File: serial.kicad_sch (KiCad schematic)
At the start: 17 parts, among them U15 LM79L05AC, U3 AM26LV32, U5 AM26LV32, U6 AM26LS30, U7 AM26LS30, U8 Am85C80

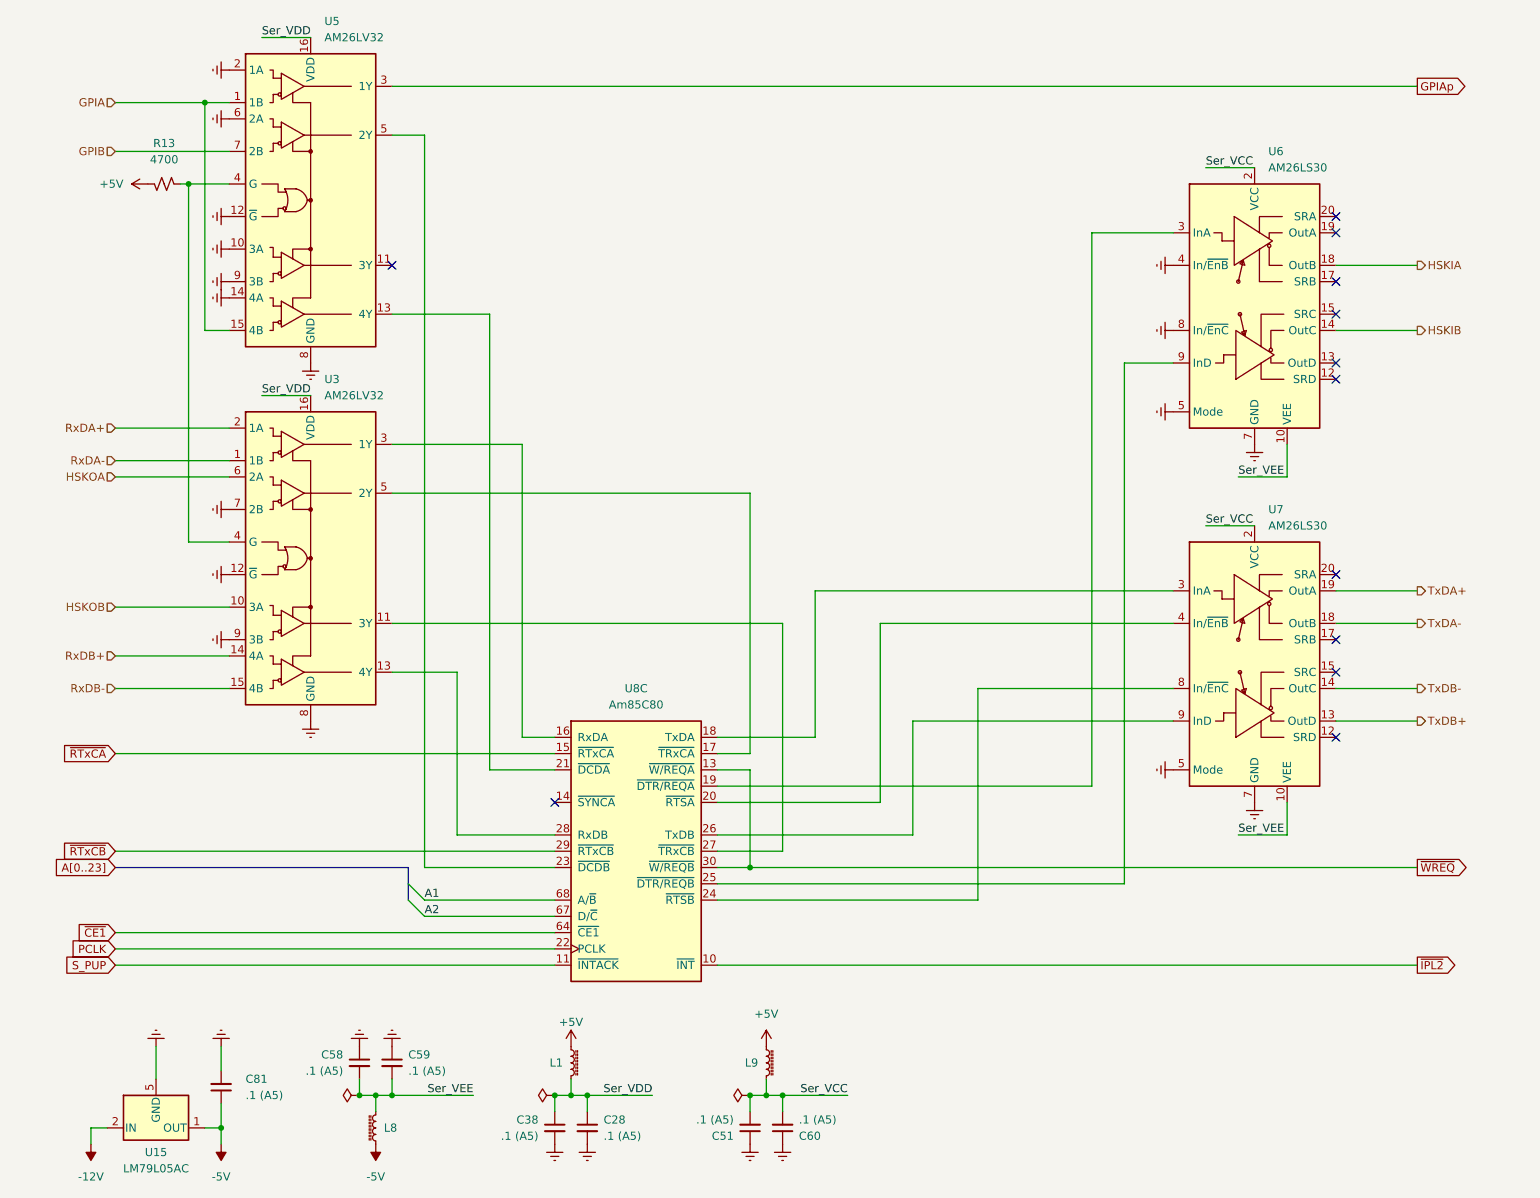
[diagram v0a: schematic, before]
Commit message: More cleanup and cosmetic fixes
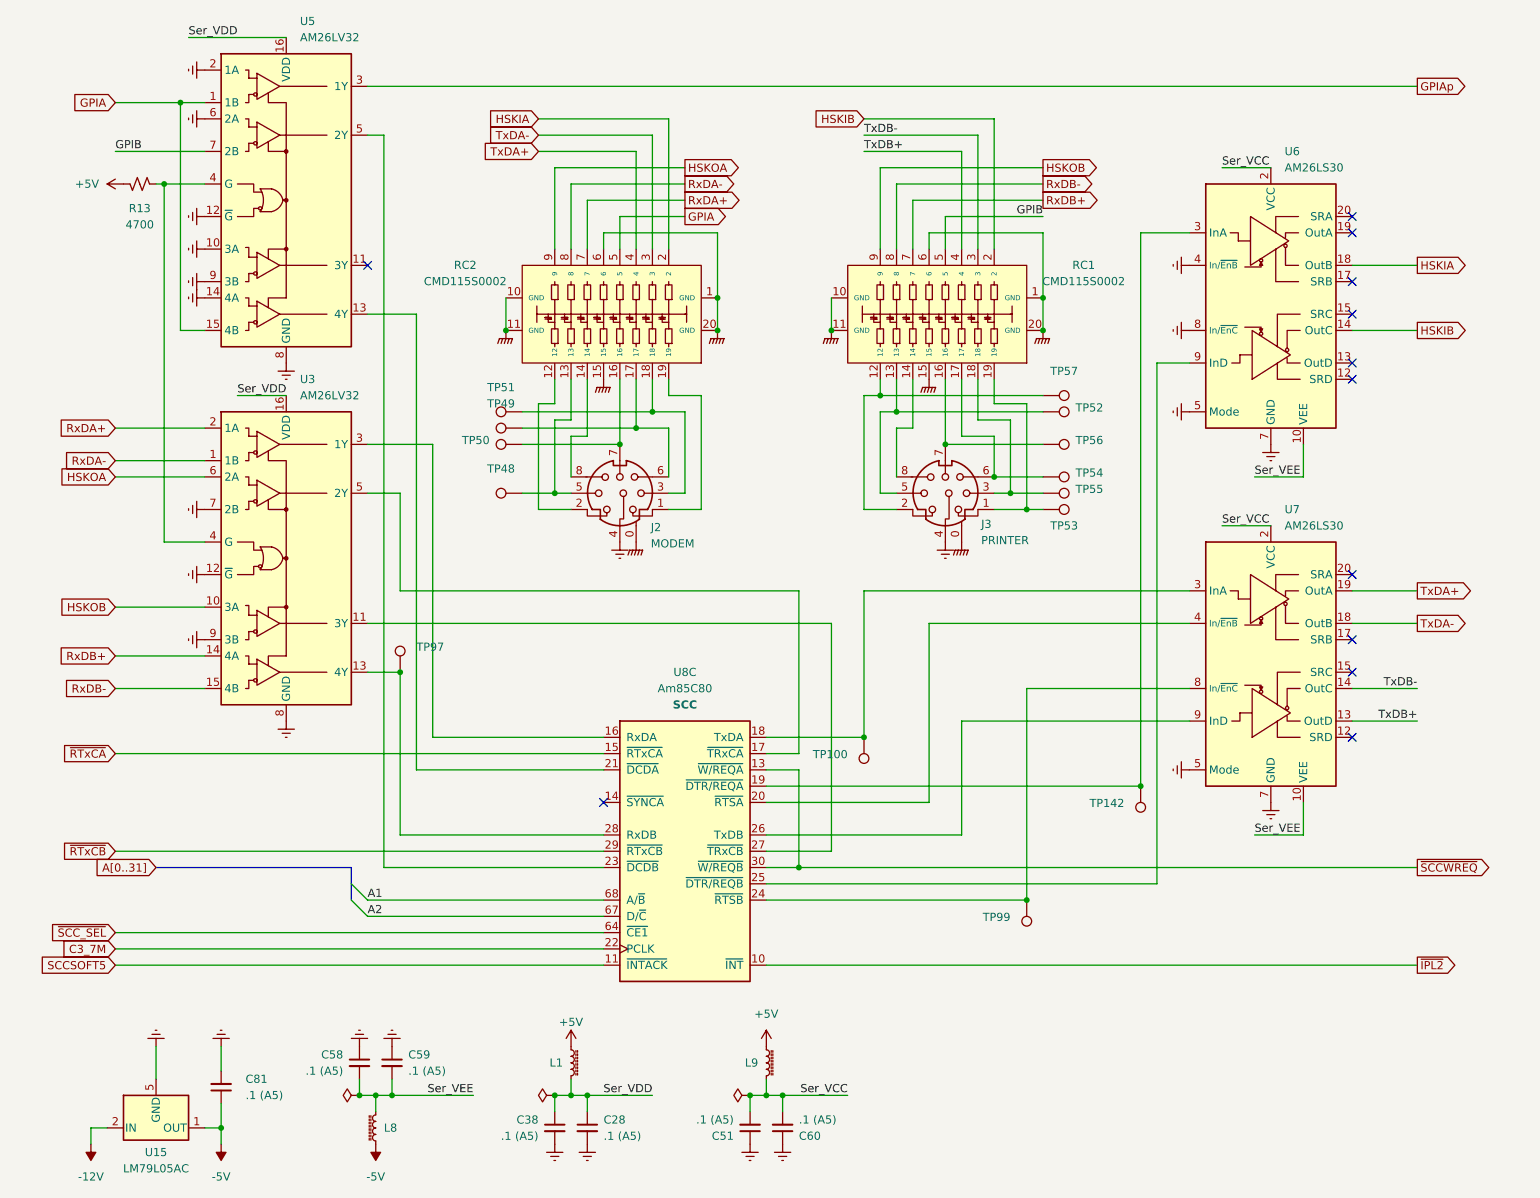
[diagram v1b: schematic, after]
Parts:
- added J2: MODEM, Connector_Imports:TE_5749268-1_MINI_DIN_8_RA_Shield, symbol MyConnector:Mini-DIN-8_MountingHole
- added J3: PRINTER, Connector_Imports:TE_5749268-1_MINI_DIN_8_RA_Shield, symbol MyConnector:Mini-DIN-8_MountingHole
- added RC1, RC2: CMD115S0002, MyPackage:SOIC-20W_7.5x12.8mm_P1.27mm_RC, symbol AppleASIC:RC_Network
- added TP100, TP142, TP48, TP49, TP50, TP51, TP52, TP53, TP54, TP55, TP56, TP57, TP97, TP99: ~, MyPackage:TestPoint_THTPad_D1.0mm_Drill0.5mm, symbol Connector:TestPoint
- U8: Desc (none) -> SCC; Desc2 (none) -> SCSI
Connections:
- net GND: now also J2.4, J3.4
- net GPIA: now also RC2.5
- net GPIB: now also RC1.5
- net HSKIA: now also RC2.2
- net HSKIB: now also RC1.2
- net HSKOA: now also RC2.9
- net HSKOB: now also RC1.9
- net RxDA+: now also RC2.7
- net RxDA-: now also RC2.8
- net RxDB+: now also RC1.7
- net RxDB-: now also RC1.8
- net TxDA+: now also RC2.4
- net TxDA-: now also RC2.3
- net TxDB+: now also RC1.4
- net TxDB-: now also RC1.3
- net at U6.3 (InA), U8.19 (~{DTR/REQA}): now also TP142.1
- net at U3.13 (4Y), U8.28 (RxDB): now also TP97.1
- net at U7.3 (InA), U8.18 (TxDA): now also TP100.1
- net at U7.8 (In/~{EnC}), U8.24 (~{RTSB}): now also TP99.1
- net PCLK renamed C3_7M
- net S_PUP renamed SCCSOFT5
- net ~{CE1} renamed ~{SCC_SEL}
- net ~{WREQ} renamed ~{SCCWREQ}
- new net: J2.2, RC2.12
- new net: J2.5, RC2.13, TP48.1
- new net: J2.8, RC2.14
- new net: J2.7, RC2.16, TP50.1
- new net: J2.6, RC2.17, TP49.1
- new net: J2.3, RC2.18, TP51.1
- new net: J2.1, RC2.19
- new net: J3.1, RC1.19, TP53.1
- new net: J3.2, RC1.12, TP57.1
- new net: J3.3, RC1.18, TP55.1
- new net: J3.5, RC1.13, TP52.1
- new net: J3.6, RC1.17, TP54.1
- new net: J3.7, RC1.16, TP56.1
- new net: J3.8, RC1.14
- new net GNDPWR: J2.0, J3.0, RC1.1 (GND), RC1.10 (GND), RC1.11 (GND), RC1.15, RC1.20 (GND), RC1.6, RC2.1 (GND), RC2.10 (GND), RC2.11 (GND), RC2.15, RC2.20 (GND), RC2.6
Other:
- moved on the sheet: R13, U3, U5, U6, U7, U8C
